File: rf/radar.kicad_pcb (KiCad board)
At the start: 4 copper layers, 52 x 68 mm, 137 parts, among them J101 Conn_01x03, J102 Conn_Coaxial, J103 Conn_01x04, J104 Conn_01x03, J105 Conn_01x03, J106 Conn_Coaxial, J107 Conn_01x02, J801 Conn_01x02, T401 2450BL15B100, T402 2450BL15B050, U101 CP0402Q5425ENTR, U201 MAX2750, U202 MC2016K30.0000C16ESH, U203 ADF4153A, U301 QPA5219, U401 AD8343, U501 MGA-645T6, U502 MGA-645T6, U601 TLV4172, U701 SN74LV1T34, U702 SN74LV1T34, U801 ADP150AUJZ-1.8-R7, U802 LM340MPX-5.0/NOPB, U803 L78L33ABU, U804 TPS54308

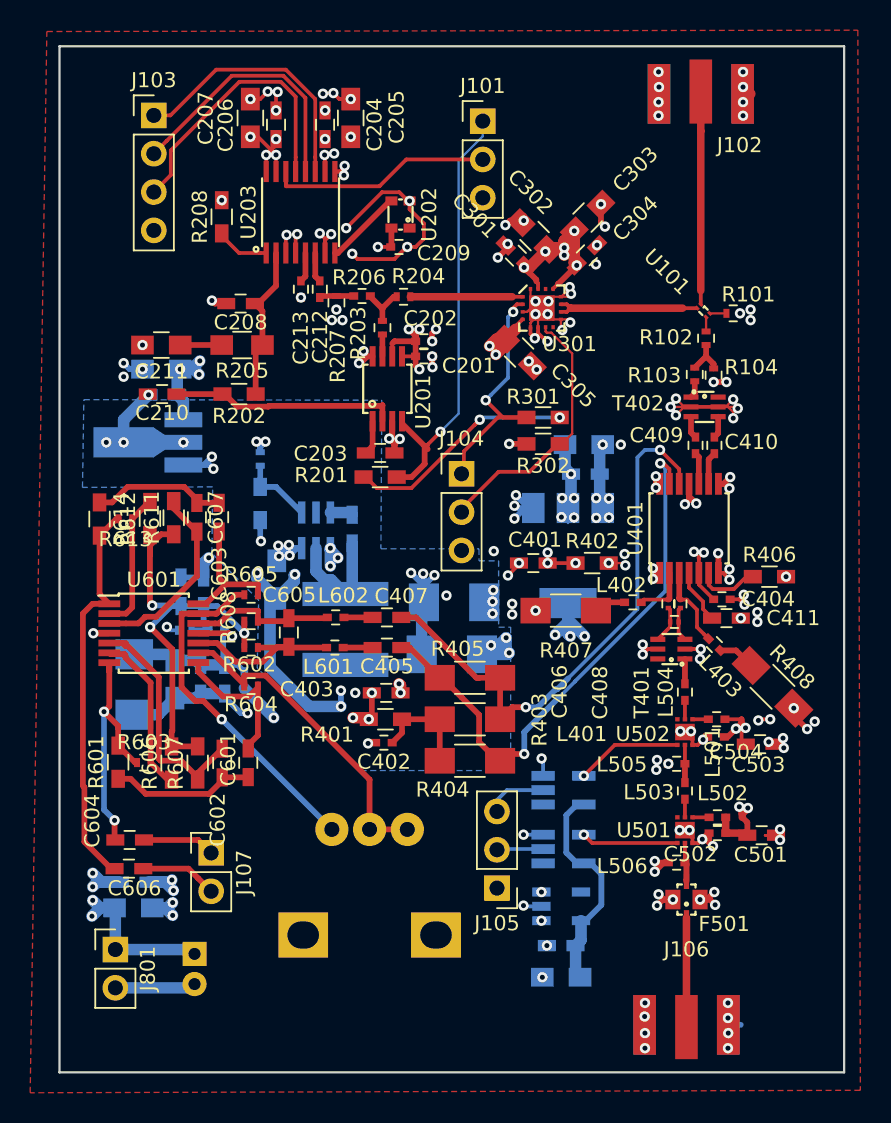
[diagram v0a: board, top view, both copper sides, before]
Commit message: Improve layout slightly
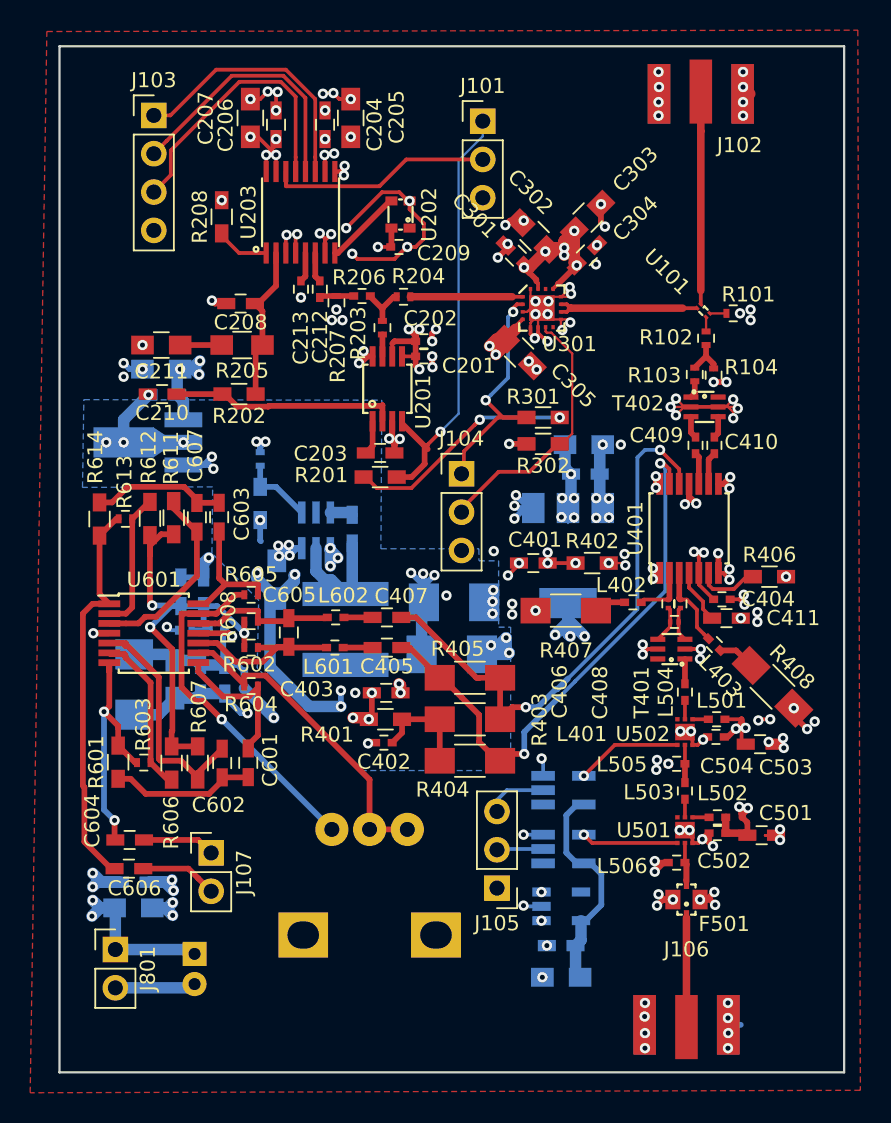
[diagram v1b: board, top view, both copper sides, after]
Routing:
- net GND: track 853.7 -> 855.2 mm
- net +12VA: track 83.7 -> 84.7 mm
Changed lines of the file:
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@@
     (thickness 1.6)
     (drawings 4)
-    (tracks 1796)
+    (tracks 1800)
     (zones 0)
     (modules 137)
@@
   )
   (setup
-    (last_trace_width 0.1524)
+    (last_trace_width 0.762)
     (user_trace_width 0.25)
     (user_trace_width 0.381)
@@
     (tags "capacitor 0603")
     (attr smd)
-    (fp_text reference C607 (at 0 -1.25 270) (layer F.SilkS)
+    (fp_text reference C607 (at -4.1021 0.1143 270) (layer F.SilkS)
       (effects (font (size 1 1) (thickness 0.15)))
     )
@@
     (tags "capacitor 0603")
     (attr smd)
-    (fp_text reference C501 (at -0.0675 1.2938) (layer F.SilkS)
+    (fp_text reference C501 (at 1.5977 -1.4732) (layer F.SilkS)
       (effects (font (size 1 1) (thickness 0.15)))
     )
@@
     (tags "capacitor 0402")
     (attr smd)
-    (fp_text reference C502 (at 1.7867 -1.3924 180) (layer F.SilkS)
+    (fp_text reference C502 (at -0.4445 -1.8415 360) (layer F.SilkS)
       (effects (font (size 1 1) (thickness 0.15)))
     )
@@
     (tags "capacitor 0603")
     (attr smd)
-    (fp_text reference C503 (at -0.1143 1.3597) (layer F.SilkS)
+    (fp_text reference C503 (at 1.7018 1.5367) (layer F.SilkS)
       (effects (font (size 1 1) (thickness 0.15)))
     )
@@
     (tags "capacitor 0402")
     (attr smd)
-    (fp_text reference C504 (at -1.3383 -1.0011 180) (layer F.SilkS)
+    (fp_text reference C504 (at -0.7151 -1.9304 180) (layer F.SilkS)
       (effects (font (size 1 1) (thickness 0.15)))
     )
@@
     (tags "capacitor 0603")
     (attr smd)
-    (fp_text reference C601 (at -0.2308 1.3285 270) (layer F.SilkS)
+    (fp_text reference C601 (at -0.1778 -1.4478 270) (layer F.SilkS)
       (effects (font (size 1 1) (thickness 0.15)))
     )
@@
     (tags "capacitor 0603")
     (attr smd)
-    (fp_text reference C602 (at -3.7622 -0.2955 90) (layer F.SilkS)
+    (fp_text reference C602 (at -2.7788 -0.2413 180) (layer F.SilkS)
       (effects (font (size 1 1) (thickness 0.15)))
     )
@@
     (tags "capacitor 0603")
     (attr smd)
-    (fp_text reference C603 (at -3.7487 0.0051 90) (layer F.SilkS)
+    (fp_text reference C603 (at 0.2057 1.4986 90) (layer F.SilkS)
       (effects (font (size 1 1) (thickness 0.15)))
     )
@@
     (tags "capacitor 0402")
     (attr smd)
-    (fp_text reference L501 (at 0.2559 -2.1993 270) (layer F.SilkS)
+    (fp_text reference L501 (at -0.3283 1.2297 360) (layer F.SilkS)
       (effects (font (size 1 1) (thickness 0.15)))
     )
@@
     (tags "resistor 0402")
     (attr smd)
-    (fp_text reference R603 (at 0 -1.35) (layer F.SilkS)
+    (fp_text reference R603 (at -0.0381 -2.5273 90) (layer F.SilkS)
       (effects (font (size 1 1) (thickness 0.15)))
     )
@@
     (tags "resistor 0603")
     (attr smd)
-    (fp_text reference R606 (at 0 -1.45 90) (layer F.SilkS)
+    (fp_text reference R606 (at -3.9448 -0.0254 90) (layer F.SilkS)
       (effects (font (size 1 1) (thickness 0.15)))
     )
@@
     (tags "resistor 0603")
     (attr smd)
-    (fp_text reference R607 (at 0 -1.45 90) (layer F.SilkS)
+    (fp_text reference R607 (at 3.7465 0.0762 90) (layer F.SilkS)
       (effects (font (size 1 1) (thickness 0.15)))
     )
@@
     (tags "resistor 0603")
     (attr smd)
-    (fp_text reference R611 (at 0 -1.45 90) (layer F.SilkS)
+    (fp_text reference R611 (at 3.9624 -0.1778 90) (layer F.SilkS)
       (effects (font (size 1 1) (thickness 0.15)))
     )
@@
     (tags "resistor 0603")
     (attr smd)
-    (fp_text reference R612 (at 0 -1.45 90) (layer F.SilkS)
+    (fp_text reference R612 (at 4.0689 -0.0889 90) (layer F.SilkS)
       (effects (font (size 1 1) (thickness 0.15)))
     )
@@
     (tags "resistor 0402")
     (attr smd)
-    (fp_text reference R613 (at 0 -1.35 180) (layer F.SilkS)
+    (fp_text reference R613 (at 0.0635 2.4384 270) (layer F.SilkS)
       (effects (font (size 1 1) (thickness 0.15)))
     )
@@
     (tags "resistor 0603")
     (attr smd)
-    (fp_text reference R614 (at 0 -1.45 270) (layer F.SilkS)
+    (fp_text reference R614 (at -4.1021 0.2794 270) (layer F.SilkS)
       (effects (font (size 1 1) (thickness 0.15)))
     )
@@
   (gr_line (start 152 100) (end 152 168) (layer Edge.Cuts) (width 0.15))
   (gr_line (start 100 100) (end 152 100) (layer Edge.Cuts) (width 0.15))
+  (segment (start 111.25 134.9) (end 113.35 132.8) (width 0.762) (layer In1.Cu) (net 1))
+  (segment (start 113.35 132.8) (end 113.338 132.8) (width 0.762) (layer In1.Cu) (net 1))
+  (segment (start 113.338 132.8) (end 113.3 132.762) (width 0.762) (layer In1.Cu) (net 1))
+  (segment (start 113.3 132.762) (end 113.3 131.4) (width 0.762) (layer In1.Cu) (net 1))
+  (via (at 113.3 131.4) (size 0.6858) (drill 0.3302) (layers F.Cu B.Cu) (net 1))
   (segment (start 143.0489 152.146) (end 143.004 152.146) (width 0.4) (layer F.Cu) (net 1))
   (segment (start 143.004 152.146) (end 142.6 152.55) (width 0.4) (layer F.Cu) (net 1))
@@
   (segment (start 113.465067 135.75) (end 113.5 135.75) (width 0.762) (layer In1.Cu) (net 1))
   (segment (start 110.4 135.75) (end 111.25 134.9) (width 0.762) (layer In1.Cu) (net 1))
-  (segment (start 111.25 134.9) (end 111.55 134.6) (width 0.762) (layer In1.Cu) (net 1))
   (segment (start 129.265406 133.456934) (end 128.780473 133.456934) (width 0.762) (layer In1.Cu) (net 1))
   (segment (start 128.29554 133.456934) (end 128.780473 133.456934) (width 0.381) (layer In1.Cu) (net 1))
@@
   (segment (start 118.65 143.75) (end 118.65 142.7) (width 0.381) (layer B.Cu) (net 1))
   (via (at 118.65 142.7) (size 0.6858) (drill 0.3302) (layers F.Cu B.Cu) (net 1))
-  (segment (start 111.55 134.6) (end 113.35 132.8) (width 0.762) (layer In1.Cu) (net 1))
   (segment (start 109.06071 140.6) (end 109.06071 137.08929) (width 0.762) (layer In1.Cu) (net 1))
   (segment (start 106.2 160.53137) (end 106.2 159.2) (width 0.762) (layer In1.Cu) (net 1))
@@
   (via (at 133.85 118.3) (size 0.6858) (drill 0.3302) (layers F.Cu B.Cu) (net 1))
   (via (at 120.45 146.2) (size 0.6858) (drill 0.3302) (layers F.Cu B.Cu) (net 1))
-  (via (at 113.35 132.8) (size 0.6858) (drill 0.3302) (layers F.Cu B.Cu) (net 1))
   (via (at 102.24051 138.9) (size 0.6858) (drill 0.3302) (layers F.Cu B.Cu) (net 1))
   (via (at 132.35 117.75) (size 0.6858) (drill 0.3302) (layers F.Cu B.Cu) (net 1))
@@
   (segment (start 123.3 141) (end 124 140.3) (width 0.762) (layer B.Cu) (net 23))
   (segment (start 118.95 141) (end 120 141) (width 0.762) (layer B.Cu) (net 23))
+  (segment (start 115.2 133.05) (end 115.2 133.15) (width 0.762) (layer In2.Cu) (net 24))
+  (segment (start 115.2 133.15) (end 114.55 133.8) (width 0.762) (layer In2.Cu) (net 24))
   (via (at 114.2 144.5) (size 0.6858) (drill 0.3302) (layers F.Cu B.Cu) (net 24))
   (segment (start 103.7 154.357101) (end 102.642899 154.357101) (width 0.762) (layer In2.Cu) (net 24))
@@
     (polygon
       (pts
-        (xy 102 157.8) (xy 102 161) (xy 110.2 161) (xy 114 157.2) (xy 114 146.2)
-        (xy 115 145.2) (xy 115 134) (xy 115 132.6) (xy 112.6 132.6) (xy 109.6 135.6)
+        (xy 102 157.8) (xy 102 161) (xy 110.2 161) (xy 114 157.2) (xy 114.9858 156.1973)
+        (xy 115 145.2) (xy 115 134) (xy 115 132.6) (xy 109.601 132.6515) (xy 109.6 135.6)
         (xy 109.6 144.8) (xy 102 152.8)
       )
